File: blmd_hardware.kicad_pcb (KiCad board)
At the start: 4 copper layers, 50 x 28.5 mm, 77 parts, among them J1 MR30PW-F, J2 control, J3 GND, J4 12V, J5 STLink-V3, Q1 RH6L040BG, Q2 RH6L040BG, Q3 RH6L040BG, Q4 RH6L040BG, Q5 RH6L040BG, Q6 RH6L040BG, SW1 reset, SW2 KHS42E, U1 LM5106MMX_NOPB, U10 STM32G431KBTx, U2 LM5106MMX_NOPB, U3 LM5106MMX_NOPB, U4 SI8620BB-B-IS, U5 SI8620BB-B-IS, U6 ACS711KEXLT-31AB, U7 ACS711KEXLT-31AB, U8 BD950N1G-C, U9 BD41041FJ-C

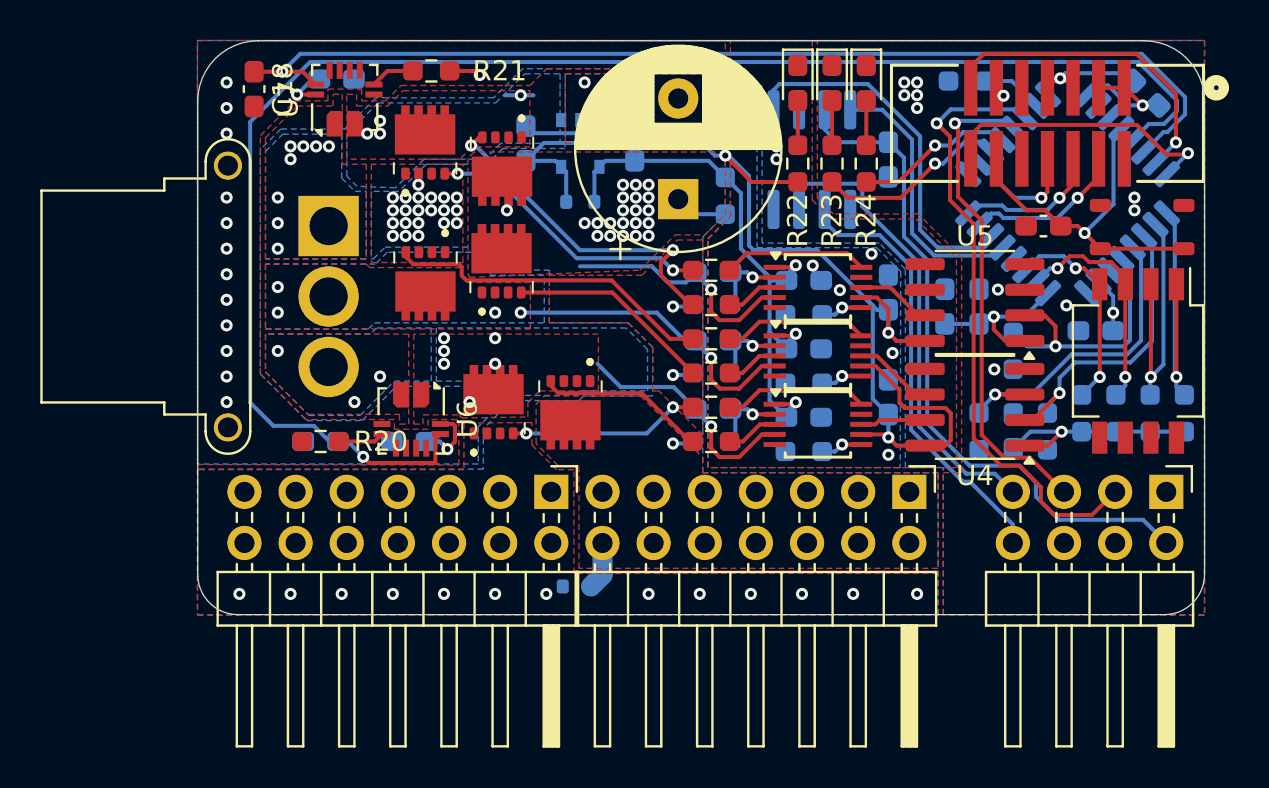
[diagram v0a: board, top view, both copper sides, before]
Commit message: back up commit
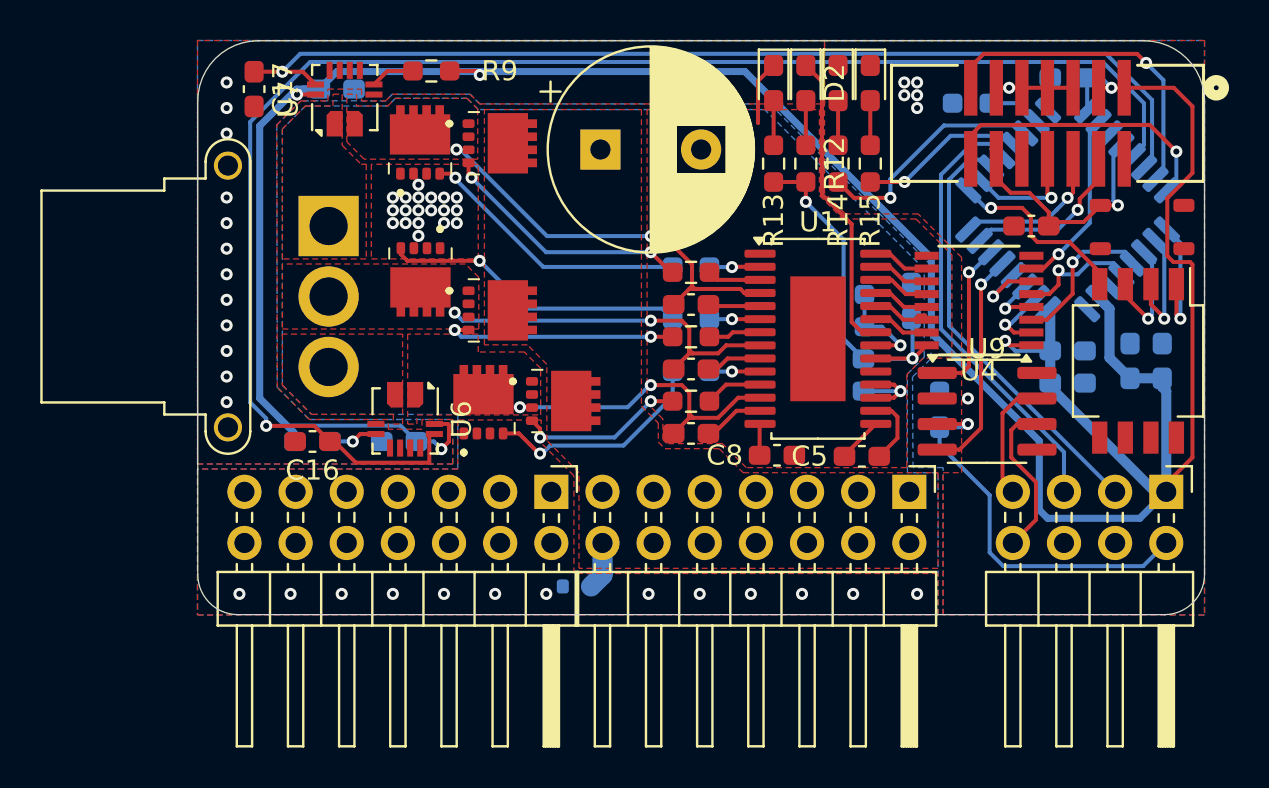
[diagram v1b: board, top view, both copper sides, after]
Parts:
- removed the C19 at (71.7, 55.1)
- removed C20: 0.1u, Capacitor_SMD:C_0603_1608Metric_Pad1.08x0.95mm_HandSolder
- removed the C9 at (84.3, 62.5)
- removed the D3 at (75.6, 66.6)
- removed the D4 at (75.6, 63.2)
- removed the D5 at (69.0, 58.0)
- removed the R1 at (76.2, 57.7)
- removed the R10 at (80.1, 67.0)
- removed the R11 at (80.1, 63.6)
- removed the R13 at (88.8, 69.4)
- removed the R14 at (90.5, 65.4)
- removed the R15 at (99.0, 68.5)
- removed R16, R17, R18: 10k, Resistor_SMD:R_0603_1608Metric_Pad0.98x0.95mm_HandSolder
- removed the R2 at (76.2, 53.7)
- removed the R9 at (80.1, 70.4)
- removed U2, U3: LM5106MMX_NOPB, Package_SO:TSSOP-10_3x3mm_P0.5mm
- removed U5: SI8620BB-B-IS, Package_SO:SOIC-8_3.9x4.9mm_P1.27mm
- removed U8: BD950N1G-C, Package_SO:TSOP-5_1.65x3.05mm_P0.95mm
- added C7: 0.22u, Capacitor_SMD:C_0603_1608Metric_Pad1.08x0.95mm_HandSolder, B.Cu at (82.2, 67.4)
- added R7: 15k, Resistor_SMD:R_0603_1608Metric_Pad0.98x0.95mm_HandSolder, B.Cu at (82.2, 64.2)
- added R8: 10k, Resistor_SMD:R_0603_1608Metric_Pad0.98x0.95mm_HandSolder, B.Cu at (82.2, 62.6)
- C16: renamed from C17; moved to F.Cu
- C2, U9: moved to F.Cu
- C3: renamed from C4; moved to F.Cu
- C4: renamed from C3; moved to F.Cu
- C5: renamed from C7; moved to F.Cu
- C6: value 0.47u -> 1u
- C8: renamed from C5; value 0.47u -> 10u; moved to F.Cu
- D2: value D -> blue; footprint Diode_SMD:D_SOD-323F -> LED_SMD:LED_0603_1608Metric_Pad1.05x0.95mm_HandSolder; moved to F.Cu
- R10: renamed from R20; moved to B.Cu
- R12: value 10k -> 2.2k; moved to F.Cu
- R2: renamed from R6; moved to B.Cu
- R4: renamed from R7; moved to B.Cu
- R6: renamed from R8; moved to B.Cu
- U1: value LM5106MMX_NOPB -> A4939KLPTR-5-T; footprint Package_SO:TSSOP-10_3x3mm_P0.5mm -> Package_SO:HTSSOP-28-1EP_4.4x9.7mm_P0.65mm_EP2.75x6.2mm
- U4: value SI8620BB-B-IS -> ISO7760FDBQR; footprint Package_SO:SOIC-8_3.9x4.9mm_P1.27mm -> Package_SO:SSOP-16_3.9x4.9mm_P0.635mm
- moved D2 18.5 mm to (80.2, 52.1), turned to -90 degrees
- moved R12 17.9 mm to (80.2, 56.1)
- moved U9 15.2 mm to (89.2, 68.4), turned to 0 degrees
- moved C19 12.7 mm to (86.8, 68.3), turned to 90 degrees
- moved C12 11.1 mm to (97.9, 65.9)
- moved C5 9.20 mm to (83.0, 70.6), turned to 180 degrees
- moved Q2 5.97 mm to (67.8, 63.4), turned to -90 degrees
- moved C10 5.81 mm to (93.2, 67.0), turned to 0 degrees
- moved U4 5.30 mm to (88.8, 62.9)
- moved Q3 4.94 mm to (67.8, 55.1), turned to -90 degrees
- moved C3 4.92 mm to (74.5, 66.3)
- moved C13 4.92 mm to (85.4, 62.9)
- moved C11 4.83 mm to (93.2, 65.4), turned to 0 degrees
- moved C1 4.58 mm to (70.0, 55.4), turned to 0 degrees
- moved U1 4.25 mm to (80.8, 64.8)
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- renumbered C22 to C10, C13 to C11, C10 to C12, C8 to C13, C15 to C14, C16 to C15, C18 to C17, C12 to C18, C14 to C19, C21 to C9, D6 to D3, D7 to D4, D8 to D5, R3 to R1, R19 to R11, R22 to R13, R23 to R14, R24 to R15, R4 to R3, R21 to R9
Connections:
- C13 pad 2: GND -> GNDPWR
- C2 pad 2: Net-(D2-K) -> Net-(U1-CA)
- C3 pad 1: HSC -> HSB
- C3 pad 2: Net-(D4-K) -> Net-(U1-CB)
- C4 pad 1: HSB -> HSC
- C4 pad 2: Net-(D3-K) -> Net-(U1-CC)
- C5 pad 1: +12V -> Net-(U1-CP1)
- C5 pad 2: GND -> Net-(U1-CP2)
- C6 pad 1: +12V -> +5V
- C6 pad 2: GND -> GNDPWR
- C8 pad 1: +12V -> GNDPWR
- C8 pad 2: GND -> Net-(U1-VREG)
- D2 pad 2: +12VA -> Net-(D2-A)
- D3 pad 1: GND -> GNDPWR
- J2 pad 3: SPD2 -> SPD1
- J2 pad 5: SPD1 -> SPD2
- J5 pad 1: unconnected-(J5-Pin_1-Pad1) -> +3V3
- J5 pad 9: unconnected-(J5-Pin_9-Pad9) -> GNDD
- R12 pad 1: SIGA -> Net-(D2-A)
- R12 pad 2: GNDD -> +5V
- U1 pad 1: +12V -> GNDPWR
- U1 pad 2: Net-(D2-K) -> LOC
- U1 pad 3: HOA -> HOC
- U1 pad 4: HSA -> HSC
- U1 pad 5: unconnected-(U1-NC-Pad5) -> Net-(U1-CC)
- U1 pad 6: Net-(U1-RDT) -> LOB
- U1 pad 7: +5V -> HOB
- U1 pad 8: PWMA -> HSB
- U1 pad 9: GND -> Net-(U1-CB)
- U10 pad 11: SIGA -> ID3
- U10 pad 12: SIGB -> SIGA_N
- U10 pad 13: SIGC -> SIGB_N
- U10 pad 18: ID3 -> SIGA
- U10 pad 19: ID4 -> SIGB
- U10 pad 2: unconnected-(U10-PF0-Pad2) -> SIGC_N
- U10 pad 20: unconnected-(U10-PA10-Pad20) -> SIGC
- U10 pad 25: unconnected-(U10-PA15-Pad25) -> ID4
- U10 pad 27: ID_DISP -> SPD1
- U10 pad 28: STATUS -> SPD2
- U10 pad 29: SPD1 -> STATUS
- U10 pad 30: SPD2 -> ID_DISP
- U4 pad 3: SIGB -> SIGA_N
- U4 pad 4: GNDD -> SIGB
- U4 pad 5: GND -> SIGB_N
- U4 pad 6: PWMB -> SIGC
- U4 pad 7: PWMA -> SIGC_N
- U4 pad 8: +5V -> GNDD
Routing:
- net +3V3: track 35.7 -> 148.2 mm, vias 7 -> 5
- net +5V: track 56.8 -> 21.3 mm, vias 3 -> 2
- net +12V: track 30.2 -> 0.00 mm, vias 3 -> 0
- net CANH: track 23.3 -> 6.13 mm
- net +5VD: track 34.9 -> 19.8 mm, vias 0 -> 1
- net CANL: track 22.3 -> 7.99 mm
- net SIGB: track 15.9 -> 2.85 mm
- net GND: track 12.1 -> 0.00 mm, vias 6 -> 0
- net SIGA: track 15.0 -> 3.57 mm
- net Net-(D2-K): track 4.09 -> 15.1 mm, vias 1 -> 0
- net TXD: track 18.2 -> 7.88 mm, vias 0 -> 1
- net SIGC: track 13.2 -> 3.70 mm
- net SIGC_N: track 0.00 -> 9.23 mm, vias 0 -> 1
- net SPD2: track 30.7 -> 22.2 mm, vias 1 -> 0
- net ID2: track 13.5 -> 6.03 mm
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- removed copper zone on In1.Cu, net +12VA
- removed copper zone on In1.Cu, net +3V3
- removed copper zone on B.Cu, net GND
- removed copper zone on F.Cu, net GND
- removed copper zone on In1.Cu, net GND
- removed copper zone on In2.Cu, net GND
- removed copper zone on In2.Cu, net GNDD
- removed copper zone on In1.Cu, net GNDPWR
- removed copper zone on In2.Cu, net GNDPWR
- removed copper zone on B.Cu, net HSA
- removed copper zone on B.Cu, net HSB
- removed copper zone on In1.Cu, net HSB
- removed copper zone on B.Cu, net HSC
- removed copper zone on In1.Cu, net HSC
- removed copper zone on B.Cu, net SOA
- removed copper zone on In1.Cu, net SOA
- removed copper zone on B.Cu, net SOC
- removed copper zone on In1.Cu, net SOC
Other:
- copper layers 4 -> 2
